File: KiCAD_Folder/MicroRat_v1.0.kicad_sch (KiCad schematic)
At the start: 15 parts, among them M1 Motor_DC, M2 Motor_DC, Q1 2N2219, Q2 TEFT4300, U1 LD1117S50TR_SOT223, U2 L293D, U3 HC-SR04

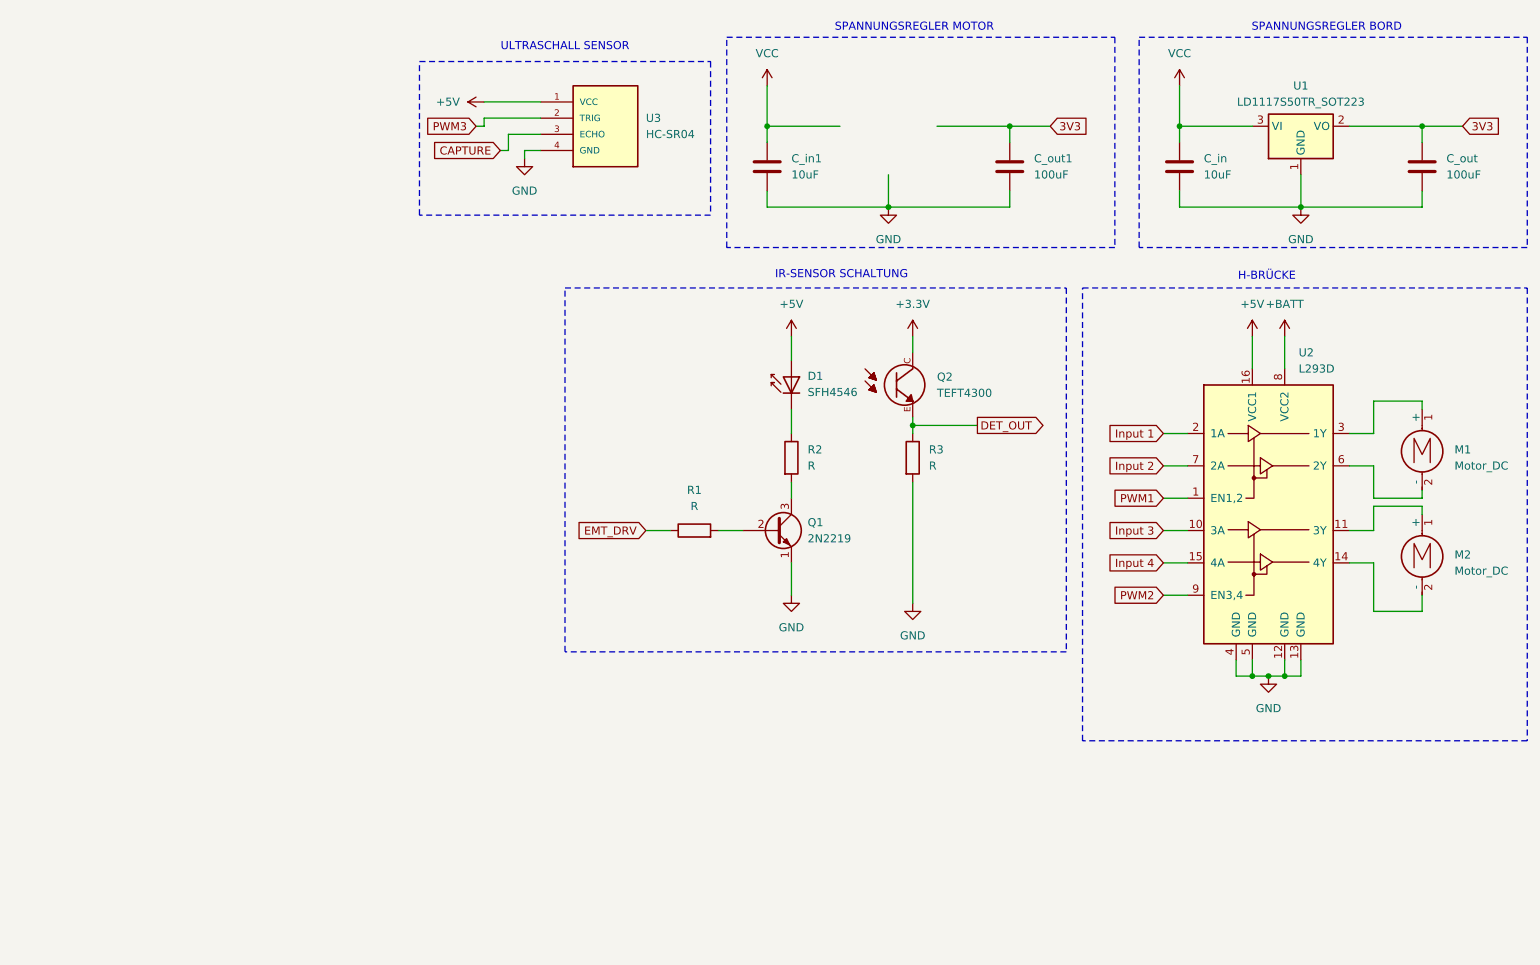
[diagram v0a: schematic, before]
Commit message: Update
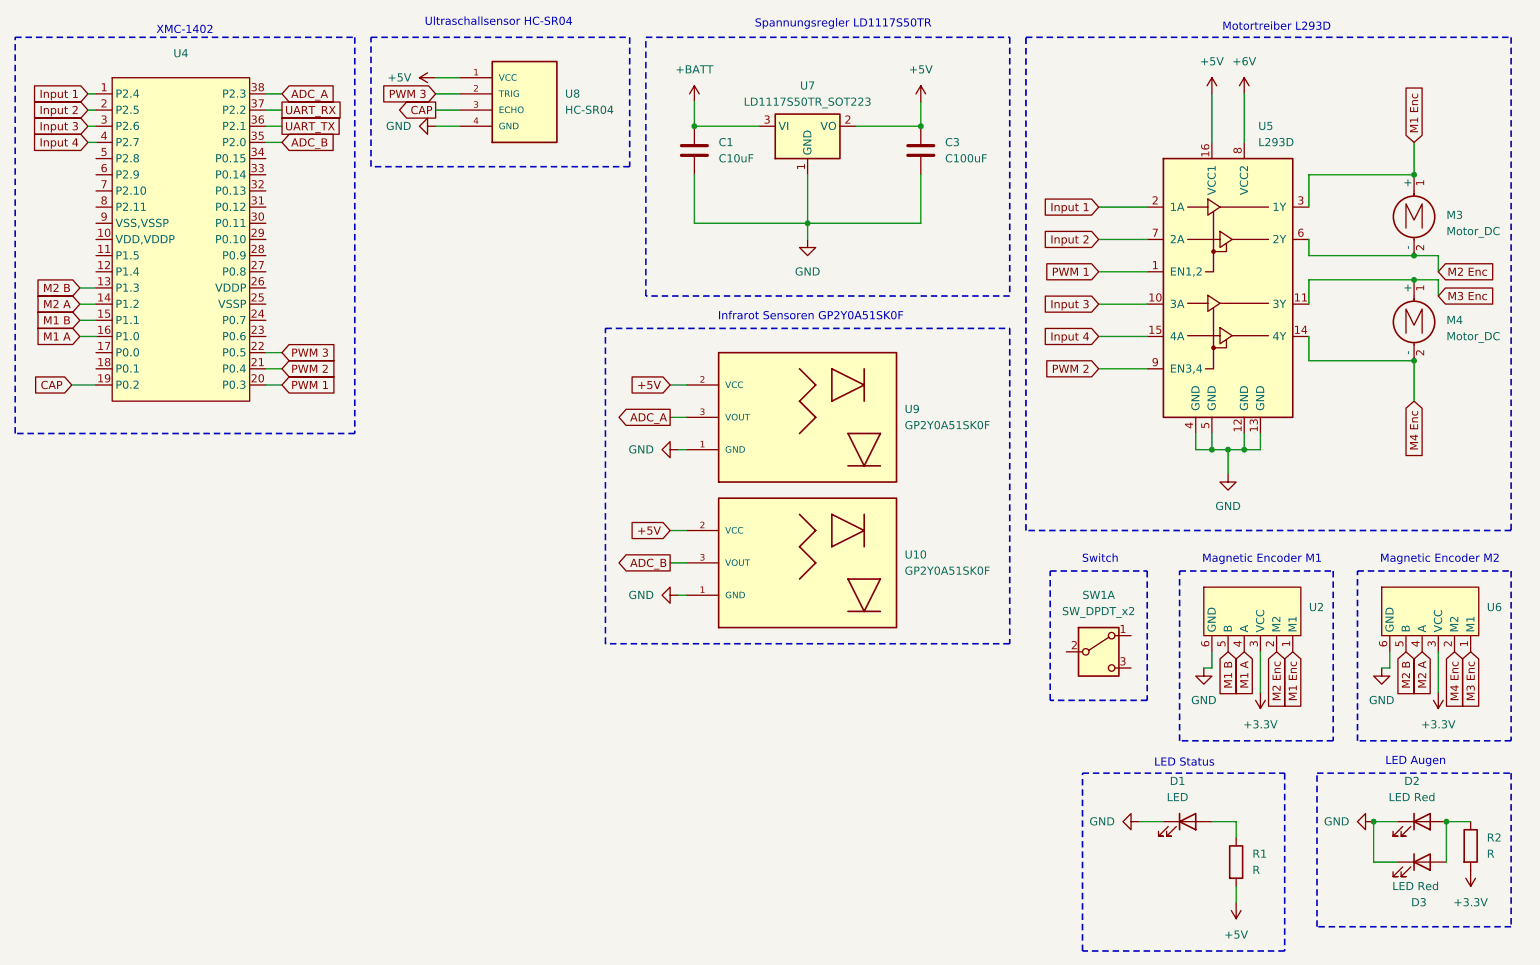
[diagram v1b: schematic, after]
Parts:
- removed C_in, C_in1: 10uF, symbol Device:C
- removed C_out, C_out1: 100uF, symbol Device:C
- removed D1: SFH4546, LED_THT:LED_D5.0mm_IRGrey, symbol LED:SFH4546
- removed M1, M2: Motor_DC, symbol Motor:Motor_DC
- removed Q1: 2N2219, Package_TO_SOT_THT:TO-39-3, symbol Transistor_BJT:2N2219
- removed Q2: TEFT4300, TEFT4300:XDCR_TEFT4300, symbol TEFT4300:TEFT4300
- removed R3: R, symbol Device:R
- removed U1: LD1117S50TR_SOT223, Package_TO_SOT_SMD:SOT-223-3_TabPin2, symbol Regulator_Linear:LD1117S50TR_SOT223
- removed U2: L293D, Package_DIP:DIP-16_W7.62mm, symbol Driver_Motor:L293D
- removed U3: HC-SR04, HC-SR04:XCVR_HC-SR04, symbol HC-SR04:HC-SR04
- added C1: C10uF, symbol Device:C
- added C3: C100uF, symbol Device:C
- added D1: LED, LED_SMD:LED_1206_3216Metric, symbol Device:LED
- added D2, D3: LED Red, symbol Device:LED
- added M3, M4: Motor_DC, symbol Motor:Motor_DC
- added SW1: SW_DPDT_x2, Button_Switch_SMD:SW_DPDT_CK_JS202011JCQN, symbol Switch:SW_DPDT_x2
- added U10, U9: GP2Y0A51SK0F, GP2Y0A21YK0F:22-23-2031, symbol GP2Y0A51SK0F:GP2Y0A21YK0F
- added U2, U6: ~, symbol New_Library:Magnetic_Encoder_1
- added U4: ~, symbol XMC1402:XMC1402
- added U5: L293D, Package_DIP:DIP-16_W7.62mm, symbol Driver_Motor:L293D
- added U7: LD1117S50TR_SOT223, Package_TO_SOT_SMD:SOT-223-3_TabPin2, symbol Regulator_Linear:LD1117S50TR_SOT223
- added U8: HC-SR04, HC-SR04:XCVR_HC-SR04, symbol HC-SR04:HC-SR04
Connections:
- net +3.3V: now also R2.2, U2.3 (VCC), U6.3 (VCC)
- net +5V: now also R1.2, C3.1, U10.2 (VCC), U5.16 (VCC1), U7.2 (VO), U8.1 (VCC), U9.2 (VCC)
- net +BATT: now also C1.1, U7.3 (VI)
- net GND: now also C1.2, C3.2, D1.1 (K), D2.1 (K), D3.1 (K), U10.1 (GND), U2.6 (GND), U5.12 (GND), U5.13 (GND), U5.4 (GND), U5.5 (GND), U6.6 (GND), U7.1 (GND), U8.4 (GND), U9.1 (GND)
- net Input 1: now also U4.1 (P2.4), U5.2 (1A)
- net Input 2: now also U4.2 (P2.5), U5.7 (2A)
- net Input 3: now also U4.3 (P2.6), U5.10 (3A)
- net Input 4: now also U4.4 (P2.7), U5.15 (4A)
- net at R2.1: now also D2.2 (A), D3.2 (A)
- net EMT_DRV: no longer names the net of R1.1
- net EMT_DRV: now also D1.2 (A)
- new net +6V: U5.8 (VCC2)
- new net ADC_A: U4.38 (P2.3), U9.3 (VOUT)
- new net ADC_B: U10.3 (VOUT), U4.35 (P2.0)
- new net CAP: U4.19 (P0.2), U8.3 (ECHO)
- new net M1 A: U2.4 (A), U4.16 (P1.0)
- new net M1 B: U2.5 (B), U4.15 (P1.1)
- new net M1 Enc: M3.1 (+), U2.1 (M1), U5.3 (1Y)
- new net M2 A: U4.14 (P1.2), U6.4 (A)
- new net M2 B: U4.13 (P1.3), U6.5 (B)
- new net M2 Enc: M3.2 (-), U2.2 (M2), U5.6 (2Y)
- new net M3 Enc: M4.1 (+), U5.11 (3Y), U6.1 (M1)
- new net M4 Enc: M4.2 (-), U5.14 (4Y), U6.2 (M2)
- new net PWM 1: U4.20 (P0.3), U5.1 (EN1,2)
- new net PWM 2: U4.21 (P0.4), U5.9 (EN3,4)
- new net PWM 3: U4.22 (P0.5), U8.2 (TRIG)
- new net UART_RX: U4.37 (P2.2)
- new net UART_TX: U4.36 (P2.1)
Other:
- note added: "Infrarot Sensoren GP2Y0A51SK0F"
- note added: "LED Augen"
- note added: "LED Status"
- note added: "Magnetic Encoder M1"
- note added: "Magnetic Encoder M2"
- note added: "Motortreiber L293D"
- note added: "Spannungsregler LD1117S50TR"
- note added: "Switch"
- note added: "Ultraschallsensor HC-SR04"
- note added: "XMC-1402"
- note removed: "H-BRÜCKE"
- note removed: "IR-SENSOR SCHALTUNG"
- note removed: "SPANNUNGSREGLER BORD"
- note removed: "SPANNUNGSREGLER MOTOR"
- note removed: "ULTRASCHALL SENSOR"
